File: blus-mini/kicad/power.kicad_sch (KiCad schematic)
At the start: 16 parts, among them U5 AMS1117-3.3, U6 AMS1117-1.8, U7 TPS54302

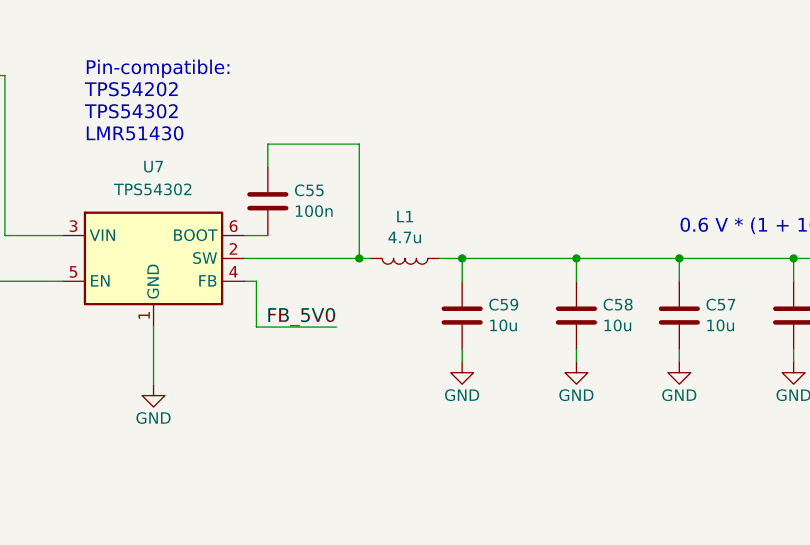
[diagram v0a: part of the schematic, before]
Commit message: chore: update submodules, minor part changes
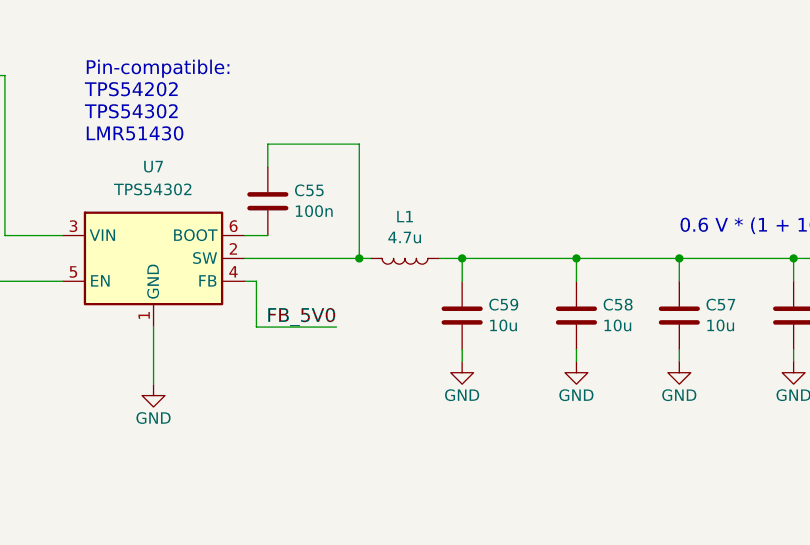
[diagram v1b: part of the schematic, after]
